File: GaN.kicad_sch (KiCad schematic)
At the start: 37 parts, among them Q1 EPC2302, Q4 EPC2302, U3 INA181A2, U7 AD8418

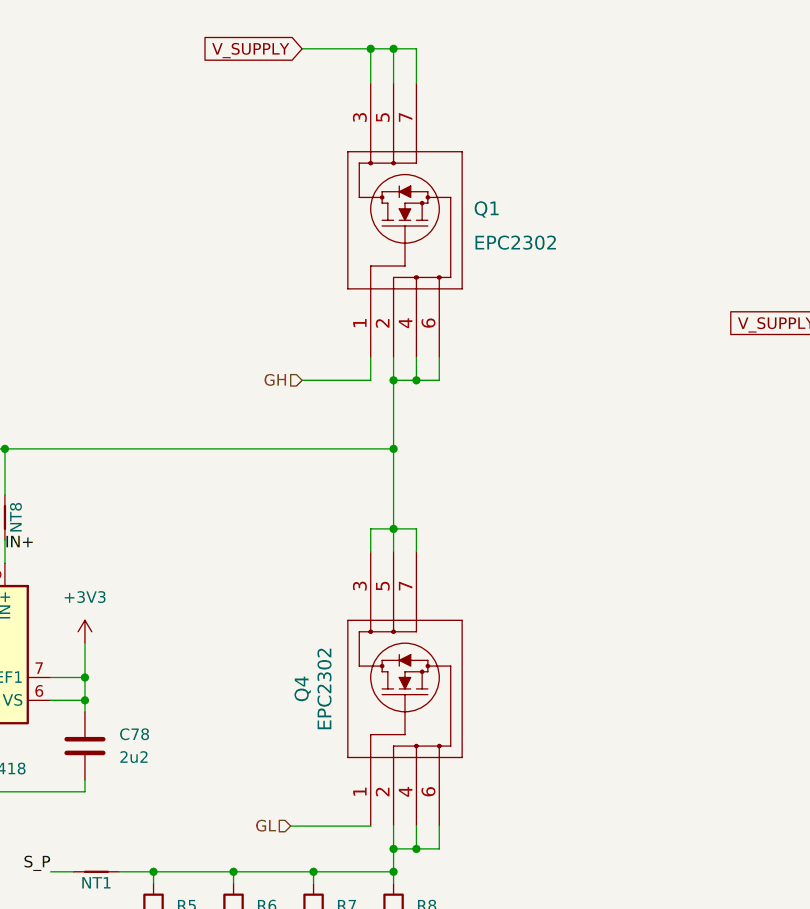
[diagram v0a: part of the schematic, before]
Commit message: update
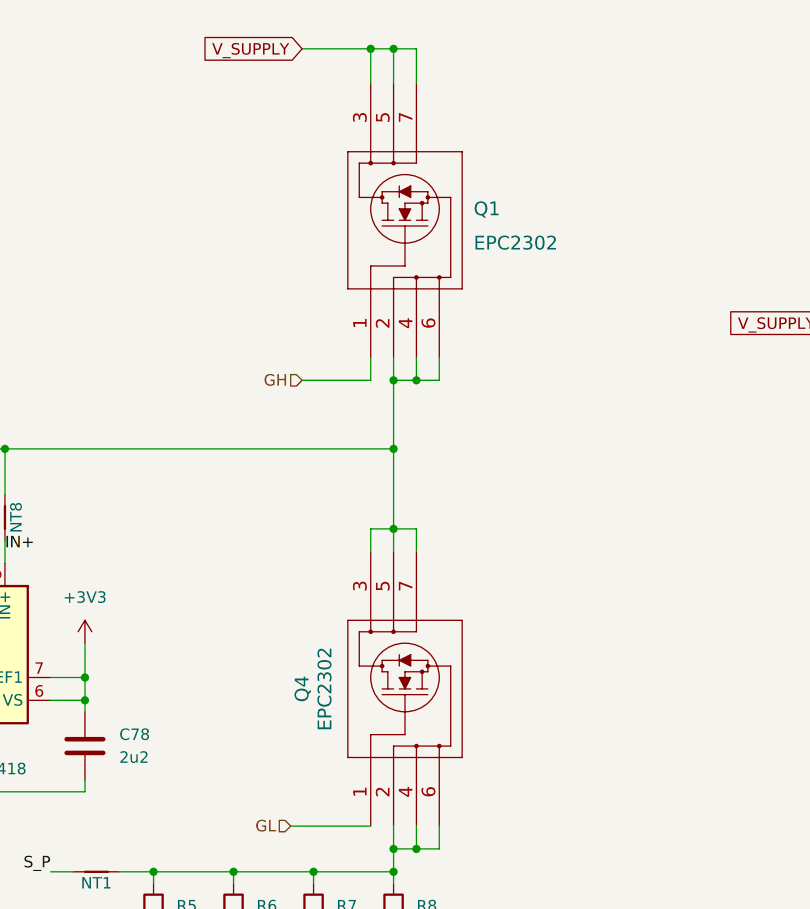
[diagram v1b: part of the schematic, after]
